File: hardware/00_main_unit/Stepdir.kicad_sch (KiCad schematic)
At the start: 2 parts, among them IC2 AM26C31CD

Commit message: Fixes after wrong merge
Signed-off-by: Jacek <matuszewski.kartech@gmail.com>
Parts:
- C26: TME C0603C104K3RAC -> (none)
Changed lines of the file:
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@@
       (effects (font (size 1.27 1.27)) hide)
     )
-    (property "TME" "C0603C104K3RAC" (id 4) (at 127 57.15 0)
+    (property "TME" "" (id 4) (at 127 57.15 0)
       (effects (font (size 1.27 1.27)) hide)
     )

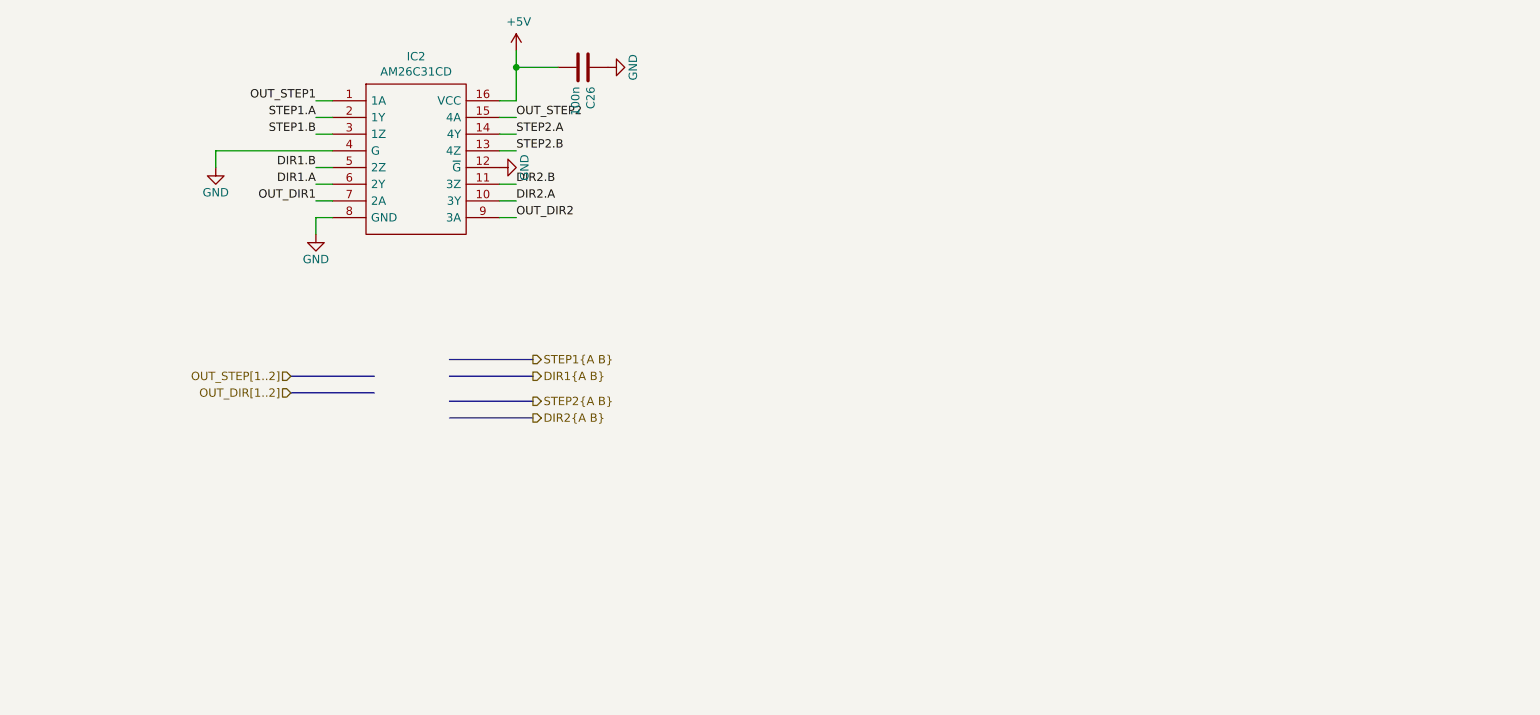
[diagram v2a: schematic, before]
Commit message: FW and SW updates for new revision
Signed-off-by: Jarosław Karwik <jaroslaw.karwik@gmail.com>
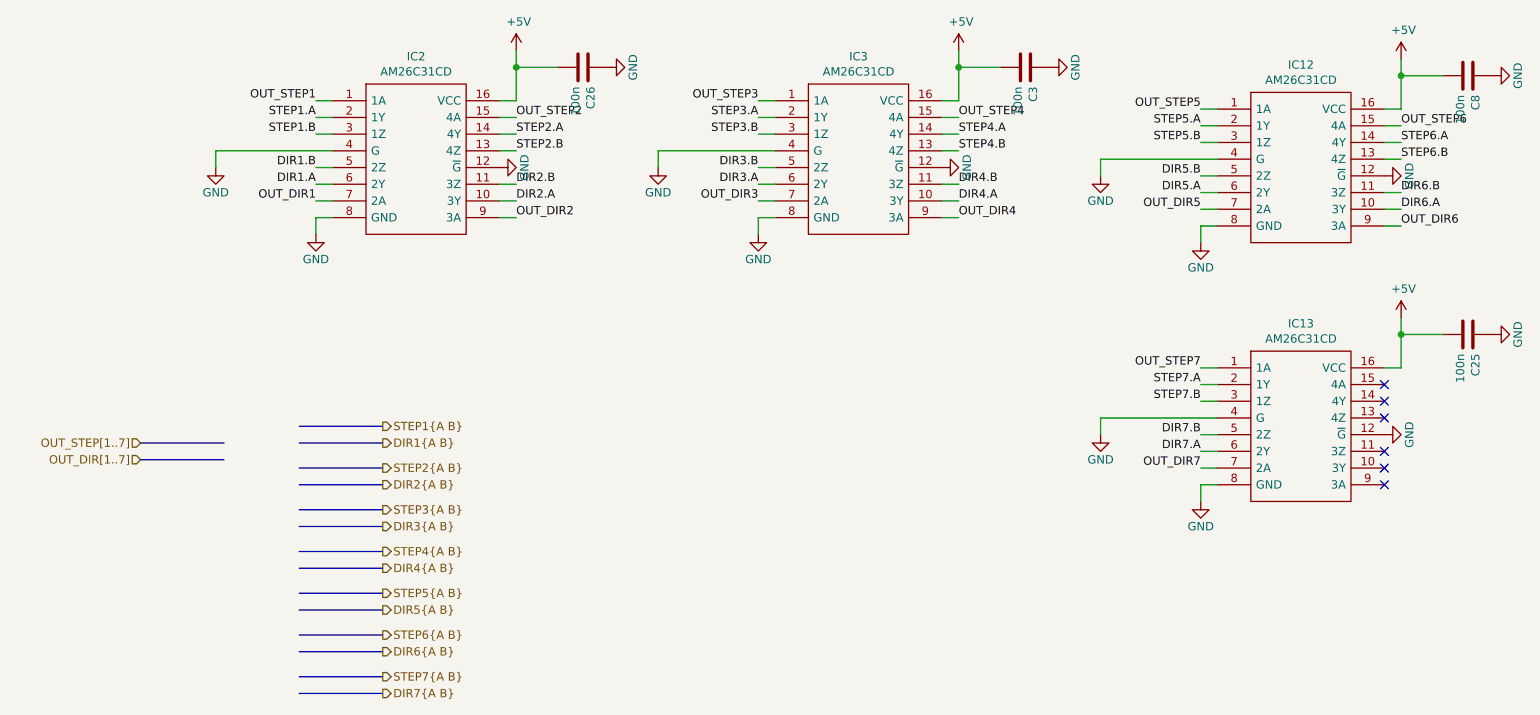
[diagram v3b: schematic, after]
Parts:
- added C25, C3, C8: 100n, Capacitor_SMD:C_0603_1608Metric, symbol Uni_Printer-rescue:C-Device
- added IC12, IC13, IC3: AM26C31CD, moje:SOIC127P600X175-16N, symbol Uni_Printer-rescue:AM26C31CD-AM26C31CD-Uni_Printer_v1-rescue
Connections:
- net +5V: now also C25.2, C3.2, C8.2, IC12.16 (VCC), IC13.16 (VCC), IC3.16 (VCC)
- net GND: now also C25.1, C3.1, C8.1, IC12.12 (~{G}), IC12.4 (G), IC12.8 (GND), IC13.12 (~{G}), IC13.4 (G), IC13.8 (GND), IC3.12 (~{G}), IC3.4 (G), IC3.8 (GND)
- new net DIR3.A: IC3.6 (2Y)
- new net DIR3.B: IC3.5 (2Z)
- new net DIR4.A: IC3.10 (3Y)
- new net DIR4.B: IC3.11 (3Z)
- new net DIR5.A: IC12.6 (2Y)
- new net DIR5.B: IC12.5 (2Z)
- new net DIR6.A: IC12.10 (3Y)
- new net DIR6.B: IC12.11 (3Z)
- new net DIR7.A: IC13.6 (2Y)
- new net DIR7.B: IC13.5 (2Z)
- new net OUT_DIR3: IC3.7 (2A)
- new net OUT_DIR4: IC3.9 (3A)
- new net OUT_DIR5: IC12.7 (2A)
- new net OUT_DIR6: IC12.9 (3A)
- new net OUT_DIR7: IC13.7 (2A)
- new net OUT_STEP3: IC3.1 (1A)
- new net OUT_STEP4: IC3.15 (4A)
- new net OUT_STEP5: IC12.1 (1A)
- new net OUT_STEP6: IC12.15 (4A)
- new net OUT_STEP7: IC13.1 (1A)
- new net STEP3.A: IC3.2 (1Y)
- new net STEP3.B: IC3.3 (1Z)
- new net STEP4.A: IC3.14 (4Y)
- new net STEP4.B: IC3.13 (4Z)
- new net STEP5.A: IC12.2 (1Y)
- new net STEP5.B: IC12.3 (1Z)
- new net STEP6.A: IC12.14 (4Y)
- new net STEP6.B: IC12.13 (4Z)
- new net STEP7.A: IC13.2 (1Y)
- new net STEP7.B: IC13.3 (1Z)
- no-connect marks 0 -> 6
